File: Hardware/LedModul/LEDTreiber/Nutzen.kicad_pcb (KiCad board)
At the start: 2 copper layers, 84 x 84 mm, 400 parts, among them J1 Conn_01x01_Pin, J2 Conn_01x01_Pin, J3 Conn_01x01_Pin, J4 Conn_01x01_Pin, J5 Conn_01x01_Pin, U1 TPS92200DxRXL, U2 TVS2700DRV

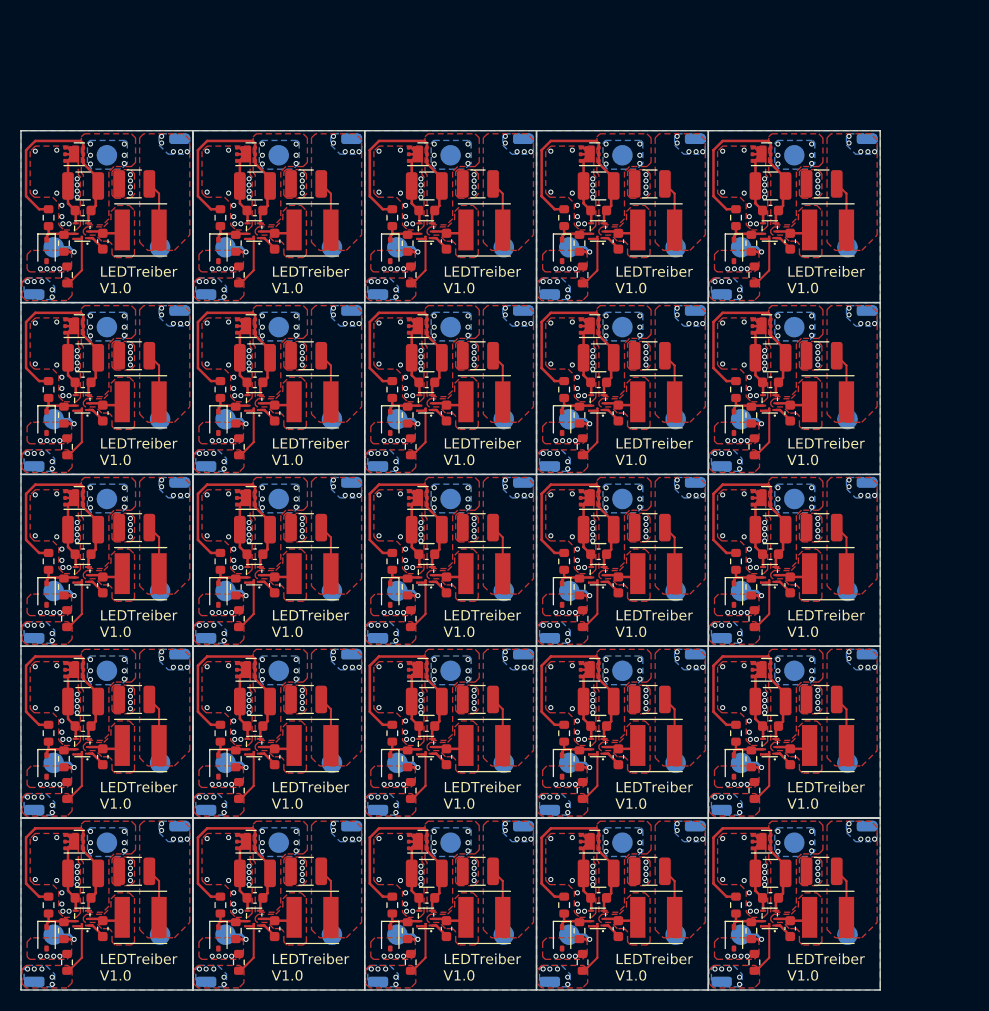
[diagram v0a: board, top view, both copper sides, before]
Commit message: V1.1
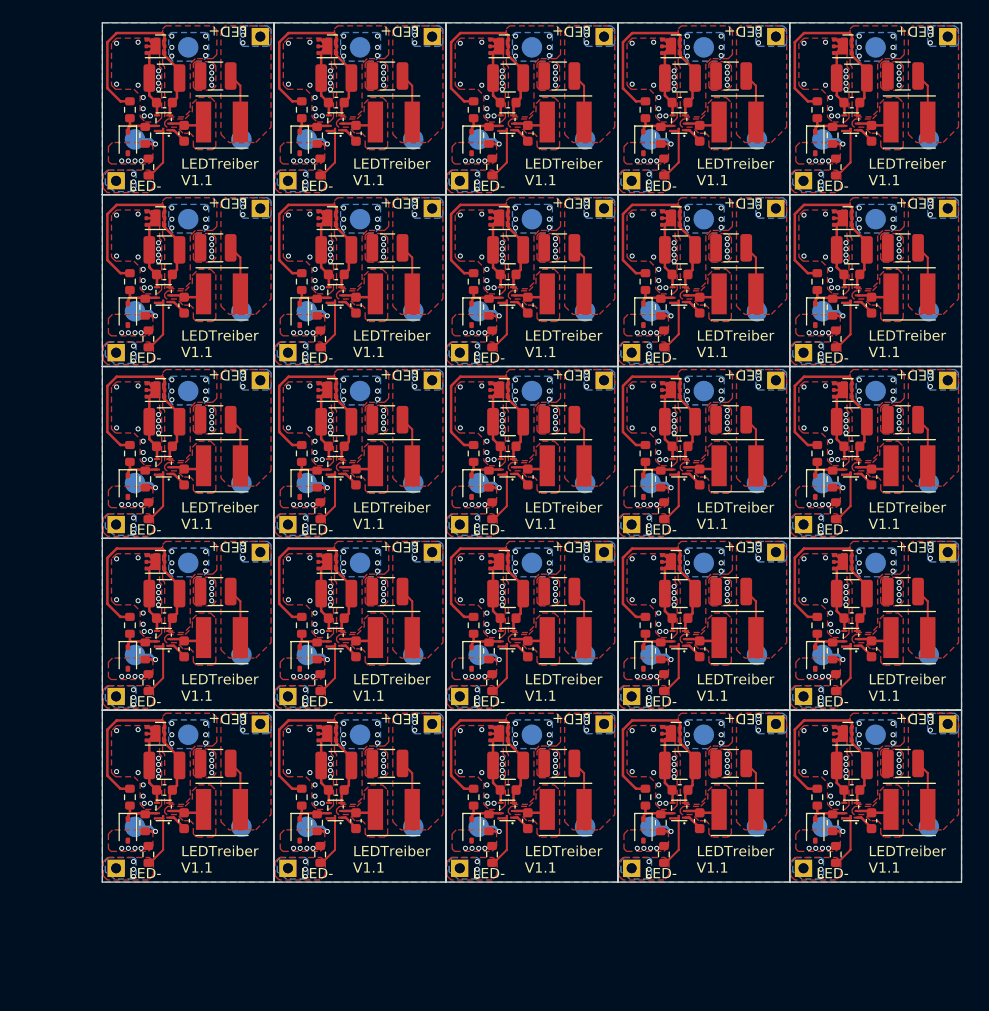
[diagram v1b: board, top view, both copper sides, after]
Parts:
- removed the C1 at (130.6, 64.8)
- removed the C1 at (97.0, 81.5)
- removed the C1 at (80.2, 115.2)
- removed the C1 at (97.0, 98.3)
- removed the C1 at (113.8, 98.3)
- removed the C1 at (147.4, 115.2)
- removed the C1 at (113.8, 64.8)
- removed the C1 at (130.6, 98.3)
- removed the C1 at (113.8, 48.0)
- removed the C1 at (80.2, 81.5)
- removed the C1 at (97.0, 64.8)
- removed the C1 at (147.4, 98.3)
- removed the C1 at (130.6, 81.5)
- removed the C1 at (147.4, 81.5)
- removed the C1 at (113.8, 115.2)
- removed the C1 at (130.6, 48.0)
- removed the C1 at (147.4, 64.8)
- removed the C1 at (147.4, 48.0)
- removed the C1 at (80.2, 98.3)
- removed the C1 at (97.0, 48.0)
- removed the C1 at (130.6, 115.2)
- removed the C1 at (80.2, 64.8)
- removed the C1 at (97.0, 115.2)
- removed the C1 at (113.8, 81.5)
- removed the C1 at (80.2, 48.0)
- removed the C2 at (110.8, 53.5)
- removed the C2 at (110.8, 120.8)
- removed the C2 at (127.5, 53.5)
- removed the C2 at (110.8, 87.2)
- removed the C2 at (110.8, 70.3)
- removed the C2 at (144.3, 53.5)
- removed the C2 at (94.0, 120.8)
- removed the C2 at (77.2, 87.2)
- removed the C2 at (77.2, 70.3)
- removed the C2 at (127.5, 104.0)
- removed the C2 at (144.3, 87.2)
- removed the C2 at (77.2, 53.5)
- removed the C2 at (94.0, 53.5)
- removed the C2 at (94.0, 104.0)
- removed the C2 at (144.3, 104.0)
- removed the C2 at (77.2, 104.0)
- removed the C2 at (127.5, 87.2)
- removed the C2 at (110.8, 104.0)
- removed the C2 at (144.3, 120.8)
- removed the C2 at (144.3, 70.3)
- removed the C2 at (94.0, 87.2)
- removed the C2 at (127.5, 70.3)
- removed the C2 at (127.5, 120.8)
- removed the C2 at (77.2, 120.8)
- removed the C2 at (94.0, 70.3)
- removed the C3 at (75.2, 115.3)
- removed the C3 at (142.4, 65.0)
- removed the C3 at (142.4, 81.8)
- removed the C3 at (75.2, 98.5)
- removed the C3 at (125.6, 98.5)
- removed the C3 at (108.8, 115.3)
- removed the C3 at (142.4, 98.5)
- removed the C3 at (75.2, 81.8)
- removed the C3 at (92.0, 98.5)
- removed the C3 at (125.6, 48.1)
- removed the C3 at (108.8, 65.0)
- removed the C3 at (142.4, 48.1)
- removed the C3 at (108.8, 81.8)
- removed the C3 at (92.0, 81.8)
- removed the C3 at (108.8, 48.1)
- removed the C3 at (125.6, 65.0)
- removed the C3 at (75.2, 48.1)
- removed the C3 at (92.0, 48.1)
- removed the C3 at (142.4, 115.3)
- removed the C3 at (125.6, 81.8)
- removed the C3 at (75.2, 65.0)
- removed the C3 at (125.6, 115.3)
- removed the C3 at (108.8, 98.5)
- removed the C3 at (92.0, 65.0)
- removed the C3 at (92.0, 115.3)
- removed the C4 at (92.0, 117.8)
- removed the C4 at (125.6, 67.3)
- removed the C4 at (142.4, 50.5)
- removed the C4 at (125.6, 101.0)
- removed the C4 at (142.4, 101.0)
- removed the C4 at (125.6, 50.5)
- removed the C4 at (108.8, 50.5)
- removed the C4 at (108.8, 84.2)
- removed the C4 at (75.2, 101.0)
- removed the C4 at (142.4, 84.2)
- removed the C4 at (142.4, 117.8)
- removed the C4 at (108.8, 67.3)
- removed the C4 at (92.0, 84.2)
- removed the C4 at (92.0, 67.3)
- removed the C4 at (75.2, 117.8)
- removed the C4 at (92.0, 101.0)
- removed the C4 at (125.6, 84.2)
- removed the C4 at (75.2, 67.3)
- removed the C4 at (75.2, 84.2)
- removed the C4 at (142.4, 67.3)
- removed the C4 at (75.2, 50.5)
- removed the C4 at (108.8, 117.8)
- removed the C4 at (108.8, 101.0)
- removed the C4 at (125.6, 117.8)
- removed the C4 at (92.0, 50.5)
- removed the D1 at (88.5, 88.0)
- removed the D1 at (71.7, 54.5)
- removed the D1 at (88.5, 71.2)
- removed the D1 at (71.7, 71.2)
- removed the D1 at (71.7, 104.8)
- removed the D1 at (88.5, 104.8)
- removed the D1 at (88.5, 54.5)
- removed the D1 at (138.8, 71.2)
- removed the D1 at (122.0, 88.0)
- removed the D1 at (88.5, 121.7)
- removed the D1 at (105.2, 121.7)
- removed the D1 at (122.0, 104.8)
- removed the D1 at (138.8, 121.7)
- removed the D1 at (71.7, 88.0)
- removed the D1 at (105.2, 71.2)
- removed the D1 at (105.2, 54.5)
- removed the D1 at (138.8, 54.5)
- removed the D1 at (122.0, 121.7)
- removed the D1 at (105.2, 88.0)
- removed the D1 at (138.8, 104.8)
- removed the D1 at (105.2, 104.8)
- removed the D1 at (122.0, 71.2)
- removed the D1 at (138.8, 88.0)
- removed the D1 at (71.7, 121.7)
- removed the D1 at (122.0, 54.5)
- removed the J1 at (118.2, 43.5)
- removed the J1 at (118.2, 110.8)
- removed the J1 at (101.5, 94.0)
- removed the J1 at (151.8, 110.8)
- removed the J1 at (84.7, 110.8)
- removed the J1 at (118.2, 60.4)
- removed the J1 at (151.8, 77.2)
- removed the J1 at (101.5, 110.8)
- removed the J1 at (135.1, 77.2)
- removed the J1 at (101.5, 60.4)
- removed the J1 at (84.7, 94.0)
- removed the J1 at (118.2, 94.0)
- removed the J1 at (151.8, 60.4)
- removed the J1 at (118.2, 77.2)
- removed the J1 at (151.8, 43.5)
- removed the J1 at (84.7, 77.2)
- removed the J1 at (101.5, 43.5)
- removed the J1 at (151.8, 94.0)
- removed the J1 at (135.1, 94.0)
- removed the J1 at (84.7, 60.4)
- removed the J1 at (135.1, 43.5)
- removed the J1 at (135.1, 110.8)
- removed the J1 at (84.7, 43.5)
- removed the J1 at (135.1, 60.4)
- removed the J1 at (101.5, 77.2)
- removed the J2 at (104.0, 58.8)
- removed the J2 at (70.5, 75.5)
- removed the J2 at (87.2, 92.3)
- removed the J2 at (104.0, 92.3)
- removed the J2 at (137.7, 126.0)
- removed the J2 at (70.5, 126.0)
- removed the J2 at (120.8, 58.8)
- removed the J2 at (104.0, 75.5)
- removed the J2 at (120.8, 75.5)
- removed the J2 at (120.8, 126.0)
- removed the J2 at (87.2, 109.2)
- removed the J2 at (137.7, 75.5)
- removed the J2 at (70.5, 58.8)
- removed the J2 at (70.5, 92.3)
- removed the J2 at (137.7, 109.2)
- removed the J2 at (120.8, 92.3)
- removed the J2 at (120.8, 109.2)
- removed the J2 at (104.0, 126.0)
- removed the J2 at (104.0, 109.2)
- removed the J2 at (87.2, 58.8)
- removed the J2 at (137.7, 58.8)
- removed the J2 at (87.2, 126.0)
- removed the J2 at (137.7, 92.3)
- removed the J2 at (87.2, 75.5)
- removed the J2 at (70.5, 109.2)
- removed the J3 at (72.3, 71.0)
- removed the J3 at (72.3, 87.8)
- removed the J3 at (89.2, 104.5)
- removed the J3 at (139.6, 54.1)
- removed the J3 at (106.0, 104.5)
- removed the J3 at (72.3, 121.3)
- removed the J3 at (106.0, 54.1)
- removed the J3 at (106.0, 121.3)
- removed the J3 at (89.2, 54.1)
- removed the J3 at (106.0, 71.0)
- removed the J3 at (89.2, 87.8)
- removed the J3 at (122.8, 104.5)
- removed the J3 at (72.3, 104.5)
- removed the J3 at (72.3, 54.1)
- removed the J3 at (139.6, 104.5)
- removed the J3 at (89.2, 121.3)
- removed the J3 at (122.8, 121.3)
- removed the J3 at (139.6, 121.3)
- removed the J3 at (122.8, 54.1)
- removed the J3 at (89.2, 71.0)
- removed the J3 at (122.8, 71.0)
- removed the J3 at (139.6, 71.0)
- removed the J3 at (139.6, 87.8)
- removed the J3 at (122.8, 87.8)
- removed the J3 at (106.0, 87.8)
- removed the J4 at (94.3, 78.8)
- removed the J4 at (144.8, 62.0)
- removed the J4 at (77.5, 95.5)
- removed the J4 at (128.0, 45.1)
- removed the J4 at (77.5, 112.3)
- removed the J4 at (77.5, 62.0)
- removed the J4 at (111.2, 62.0)
- removed the J4 at (111.2, 45.1)
- removed the J4 at (94.3, 45.1)
- removed the J4 at (128.0, 62.0)
- removed the J4 at (144.8, 95.5)
- removed the J4 at (111.2, 95.5)
- removed the J4 at (94.3, 112.3)
- removed the J4 at (94.3, 95.5)
- removed the J4 at (77.5, 78.8)
- removed the J4 at (94.3, 62.0)
- removed the J4 at (111.2, 112.3)
- removed the J4 at (128.0, 78.8)
- removed the J4 at (128.0, 95.5)
- removed the J4 at (144.8, 45.1)
- removed the J4 at (144.8, 112.3)
- removed the J4 at (128.0, 112.3)
- removed the J4 at (144.8, 78.8)
- removed the J4 at (77.5, 45.1)
- removed the J4 at (111.2, 78.8)
- removed the J5 at (82.8, 104.5)
- removed the J5 at (82.8, 54.1)
- removed the J5 at (99.5, 87.8)
- removed the J5 at (82.8, 71.0)
- removed the J5 at (116.3, 54.1)
- removed the J5 at (149.9, 71.0)
- removed the J5 at (99.5, 121.3)
- removed the J5 at (133.2, 54.1)
- removed the J5 at (82.8, 87.8)
- removed the J5 at (149.9, 121.3)
- removed the J5 at (133.2, 71.0)
- removed the J5 at (99.5, 104.5)
- removed the J5 at (133.2, 104.5)
- removed the J5 at (116.3, 104.5)
- removed the J5 at (116.3, 87.8)
- removed the J5 at (149.9, 54.1)
- removed the J5 at (99.5, 54.1)
- removed the J5 at (149.9, 87.8)
- removed the J5 at (116.3, 121.3)
- removed the J5 at (116.3, 71.0)
- removed the J5 at (99.5, 71.0)
- removed the J5 at (82.8, 121.3)
- removed the J5 at (133.2, 87.8)
- removed the J5 at (133.2, 121.3)
- removed the J5 at (149.9, 104.5)
- removed the L1 at (131.2, 86.0)
- removed the L1 at (97.7, 52.5)
- removed the L1 at (148.1, 102.8)
- removed the L1 at (80.8, 86.0)
- removed the L1 at (114.5, 86.0)
- removed the L1 at (80.8, 102.8)
- removed the L1 at (97.7, 119.7)
- removed the L1 at (148.1, 119.7)
- removed the L1 at (114.5, 69.2)
- removed the L1 at (97.7, 86.0)
- removed the L1 at (97.7, 102.8)
- removed the L1 at (114.5, 102.8)
- removed the L1 at (131.2, 69.2)
- removed the L1 at (131.2, 52.5)
- removed the L1 at (131.2, 119.7)
- removed the L1 at (148.1, 69.2)
- removed the L1 at (148.1, 52.5)
- removed the L1 at (80.8, 119.7)
- removed the L1 at (97.7, 69.2)
- removed the L1 at (114.5, 119.7)
- removed the L1 at (148.1, 86.0)
- removed the L1 at (131.2, 102.8)
- removed the L1 at (80.8, 52.5)
- removed the L1 at (114.5, 52.5)
- removed the L1 at (80.8, 69.2)
- removed the R1 at (139.1, 118.5)
- removed the R1 at (139.1, 101.7)
- removed the R1 at (88.7, 84.8)
- removed the R1 at (122.2, 51.2)
- removed the R1 at (122.2, 68.0)
- removed the R1 at (139.1, 84.8)
- removed the R1 at (71.8, 51.2)
- removed the R1 at (71.8, 118.5)
- removed the R1 at (105.5, 84.8)
- removed the R1 at (105.5, 51.2)
- removed the R1 at (139.1, 68.0)
- removed the R1 at (139.1, 51.2)
- removed the R1 at (71.8, 84.8)
- removed the R1 at (122.2, 101.7)
- removed the R1 at (122.2, 84.8)
- removed the R1 at (88.7, 51.2)
- removed the R1 at (105.5, 68.0)
- removed the R1 at (105.5, 118.5)
- removed the R1 at (88.7, 101.7)
- removed the R1 at (71.8, 101.7)
- removed the R1 at (71.8, 68.0)
- removed the R1 at (122.2, 118.5)
- removed the R1 at (88.7, 118.5)
- removed the R1 at (105.5, 101.7)
- removed the R1 at (88.7, 68.0)
- removed the R2 at (140.8, 90.5)
- removed the R2 at (73.7, 107.2)
- removed the R2 at (140.8, 107.2)
- removed the R2 at (107.2, 107.2)
- removed the R2 at (107.2, 90.5)
- removed the R2 at (107.2, 124.0)
- removed the R2 at (90.5, 73.7)
- removed the R2 at (73.7, 73.7)
- removed the R2 at (140.8, 124.0)
- removed the R2 at (90.5, 124.0)
- removed the R2 at (90.5, 56.9)
- removed the R2 at (107.2, 73.7)
- removed the R2 at (73.7, 124.0)
- removed the R2 at (90.5, 107.2)
- removed the R2 at (140.8, 73.7)
- removed the R2 at (73.7, 56.9)
- removed the R2 at (90.5, 90.5)
- removed the R2 at (73.7, 90.5)
- removed the R2 at (124.0, 56.9)
- removed the R2 at (140.8, 56.9)
- removed the R2 at (124.0, 107.2)
- removed the R2 at (124.0, 73.7)
- removed the R2 at (107.2, 56.9)
- removed the R2 at (124.0, 90.5)
- removed the R2 at (124.0, 124.0)
- removed the R3 at (107.0, 70.5)
- removed the R3 at (73.3, 121.0)
- removed the R3 at (73.3, 53.8)
- removed the R3 at (140.6, 121.0)
- removed the R3 at (90.2, 70.5)
- removed the R3 at (90.2, 104.2)
- removed the R3 at (123.8, 70.5)
- removed the R3 at (140.6, 104.2)
- removed the R3 at (140.6, 70.5)
- removed the R3 at (123.8, 104.2)
- removed the R3 at (123.8, 87.3)
- removed the R3 at (140.6, 53.8)
- removed the R3 at (90.2, 53.8)
- removed the R3 at (123.8, 53.8)
- removed the R3 at (107.0, 87.3)
- removed the R3 at (73.3, 104.2)
- removed the R3 at (107.0, 104.2)
- removed the R3 at (73.3, 70.5)
- removed the R3 at (107.0, 121.0)
- removed the R3 at (90.2, 87.3)
- removed the R3 at (123.8, 121.0)
- removed the R3 at (90.2, 121.0)
- removed the R3 at (140.6, 87.3)
- removed the R3 at (73.3, 87.3)
- removed the R3 at (107.0, 53.8)
- removed the U1 at (108.8, 69.3)
- removed the U1 at (125.5, 52.5)
- removed the U1 at (108.8, 103.0)
- removed the U1 at (142.3, 103.0)
- removed the U1 at (125.5, 86.2)
- removed the U1 at (142.3, 69.3)
- removed the U1 at (75.2, 86.2)
- removed the U1 at (92.0, 103.0)
- removed the U1 at (92.0, 52.5)
- removed the U1 at (92.0, 119.8)
- removed the U1 at (142.3, 52.5)
- removed the U1 at (75.2, 119.8)
- removed the U1 at (142.3, 86.2)
- removed the U1 at (75.2, 52.5)
- removed the U1 at (142.3, 119.8)
- removed the U1 at (75.2, 69.3)
- removed the U1 at (125.5, 119.8)
- removed the U1 at (108.8, 119.8)
- removed the U1 at (75.2, 103.0)
- removed the U1 at (92.0, 69.3)
- removed the U1 at (108.8, 86.2)
- removed the U1 at (125.5, 103.0)
- removed the U1 at (125.5, 69.3)
- removed the U1 at (92.0, 86.2)
- removed the U1 at (108.8, 52.5)
- removed the U2 at (91.2, 61.9)
- removed the U2 at (108.0, 112.2)
- removed the U2 at (91.2, 112.2)
- removed the U2 at (141.6, 112.2)
- removed the U2 at (141.6, 45.0)
- removed the U2 at (141.6, 95.5)
- removed the U2 at (124.8, 61.9)
- removed the U2 at (141.6, 78.7)
- removed the U2 at (141.6, 61.9)
- removed the U2 at (124.8, 45.0)
- removed the U2 at (108.0, 45.0)
- removed the U2 at (91.2, 95.5)
- removed the U2 at (124.8, 95.5)
- removed the U2 at (108.0, 78.7)
- removed the U2 at (91.2, 78.7)
- removed the U2 at (74.3, 61.9)
- removed the U2 at (124.8, 78.7)
- removed the U2 at (91.2, 45.0)
- removed the U2 at (108.0, 61.9)
- removed the U2 at (74.3, 78.7)
- removed the U2 at (108.0, 95.5)
- removed the U2 at (74.3, 45.0)
- removed the U2 at (124.8, 112.2)
- removed the U2 at (74.3, 95.5)
- removed the U2 at (74.3, 112.2)
- added C1: 10µ, Capacitor_SMD:C_1210_3225Metric, F.Cu at (155.4, 54.2)
- added C1: 10µ, Capacitor_SMD:C_1210_3225Metric, F.Cu at (121.8, 87.8)
- added C1: 10µ, Capacitor_SMD:C_1210_3225Metric, F.Cu at (105.0, 87.8)
- added C1: 10µ, Capacitor_SMD:C_1210_3225Metric, F.Cu at (138.6, 87.8)
- added C1: 10µ, Capacitor_SMD:C_1210_3225Metric, F.Cu at (88.2, 71.0)
- added C1: 10µ, Capacitor_SMD:C_1210_3225Metric, F.Cu at (121.8, 104.6)
- added C1: 10µ, Capacitor_SMD:C_1210_3225Metric, F.Cu at (155.4, 37.4)
- added C1: 10µ, Capacitor_SMD:C_1210_3225Metric, F.Cu at (138.6, 104.6)
- added C1: 10µ, Capacitor_SMD:C_1210_3225Metric, F.Cu at (121.8, 71.0)
- added C1: 10µ, Capacitor_SMD:C_1210_3225Metric, F.Cu at (105.0, 104.6)
- added C1: 10µ, Capacitor_SMD:C_1210_3225Metric, F.Cu at (155.4, 104.6)
- added C1: 10µ, Capacitor_SMD:C_1210_3225Metric, F.Cu at (105.0, 71.0)
- added C1: 10µ, Capacitor_SMD:C_1210_3225Metric, F.Cu at (105.0, 54.2)
- added C1: 10µ, Capacitor_SMD:C_1210_3225Metric, F.Cu at (88.2, 87.8)
- added C1: 10µ, Capacitor_SMD:C_1210_3225Metric, F.Cu at (88.2, 37.4)
- added C1: 10µ, Capacitor_SMD:C_1210_3225Metric, F.Cu at (155.4, 87.8)
- added C1: 10µ, Capacitor_SMD:C_1210_3225Metric, F.Cu at (88.2, 104.6)
- added C1: 10µ, Capacitor_SMD:C_1210_3225Metric, F.Cu at (155.4, 71.0)
- added C1: 10µ, Capacitor_SMD:C_1210_3225Metric, F.Cu at (138.6, 37.4)
- added C1: 10µ, Capacitor_SMD:C_1210_3225Metric, F.Cu at (138.6, 71.0)
- added C1: 10µ, Capacitor_SMD:C_1210_3225Metric, F.Cu at (105.0, 37.4)
- added C1: 10µ, Capacitor_SMD:C_1210_3225Metric, F.Cu at (121.8, 54.2)
- added C1: 10µ, Capacitor_SMD:C_1210_3225Metric, F.Cu at (138.6, 54.2)
- added C1: 10µ, Capacitor_SMD:C_1210_3225Metric, F.Cu at (88.2, 54.2)
- added C1: 10µ, Capacitor_SMD:C_1210_3225Metric, F.Cu at (121.8, 37.4)
- added C2: 100n, Capacitor_SMD:C_0603_1608Metric, F.Cu at (152.3, 93.4)
- added C2: 100n, Capacitor_SMD:C_0603_1608Metric, F.Cu at (101.9, 76.6)
- added C2: 100n, Capacitor_SMD:C_0603_1608Metric, F.Cu at (101.9, 110.2)
- added C2: 100n, Capacitor_SMD:C_0603_1608Metric, F.Cu at (101.9, 59.8)
- added C2: 100n, Capacitor_SMD:C_0603_1608Metric, F.Cu at (101.9, 93.4)
- added C2: 100n, Capacitor_SMD:C_0603_1608Metric, F.Cu at (135.5, 93.4)
- added C2: 100n, Capacitor_SMD:C_0603_1608Metric, F.Cu at (85.1, 93.4)
- added C2: 100n, Capacitor_SMD:C_0603_1608Metric, F.Cu at (152.3, 59.8)
- added C2: 100n, Capacitor_SMD:C_0603_1608Metric, F.Cu at (85.1, 76.6)
- added C2: 100n, Capacitor_SMD:C_0603_1608Metric, F.Cu at (85.1, 59.8)
- added C2: 100n, Capacitor_SMD:C_0603_1608Metric, F.Cu at (101.9, 43.0)
- added C2: 100n, Capacitor_SMD:C_0603_1608Metric, F.Cu at (118.7, 93.4)
- added C2: 100n, Capacitor_SMD:C_0603_1608Metric, F.Cu at (118.7, 110.2)
- added C2: 100n, Capacitor_SMD:C_0603_1608Metric, F.Cu at (135.5, 59.8)
- added C2: 100n, Capacitor_SMD:C_0603_1608Metric, F.Cu at (135.5, 110.2)
- added C2: 100n, Capacitor_SMD:C_0603_1608Metric, F.Cu at (118.7, 76.6)
- added C2: 100n, Capacitor_SMD:C_0603_1608Metric, F.Cu at (118.7, 43.0)
- added C2: 100n, Capacitor_SMD:C_0603_1608Metric, F.Cu at (135.5, 43.0)
- added C2: 100n, Capacitor_SMD:C_0603_1608Metric, F.Cu at (152.3, 110.2)
- added C2: 100n, Capacitor_SMD:C_0603_1608Metric, F.Cu at (152.3, 43.0)
- added C2: 100n, Capacitor_SMD:C_0603_1608Metric, F.Cu at (85.1, 110.2)
- added C2: 100n, Capacitor_SMD:C_0603_1608Metric, F.Cu at (85.1, 43.0)
- added C2: 100n, Capacitor_SMD:C_0603_1608Metric, F.Cu at (118.7, 59.8)
- added C2: 100n, Capacitor_SMD:C_0603_1608Metric, F.Cu at (152.3, 76.6)
- added C2: 100n, Capacitor_SMD:C_0603_1608Metric, F.Cu at (135.5, 76.6)
- added C3: 10µ, Capacitor_SMD:C_1210_3225Metric, F.Cu at (133.6, 54.4)
- added C3: 10µ, Capacitor_SMD:C_1210_3225Metric, F.Cu at (116.8, 71.2)
- added C3: 10µ, Capacitor_SMD:C_1210_3225Metric, F.Cu at (83.2, 71.2)
- added C3: 10µ, Capacitor_SMD:C_1210_3225Metric, F.Cu at (150.4, 88.0)
- added C3: 10µ, Capacitor_SMD:C_1210_3225Metric, F.Cu at (116.8, 54.4)
- added C3: 10µ, Capacitor_SMD:C_1210_3225Metric, F.Cu at (150.4, 37.6)
- added C3: 10µ, Capacitor_SMD:C_1210_3225Metric, F.Cu at (83.2, 37.6)
- added C3: 10µ, Capacitor_SMD:C_1210_3225Metric, F.Cu at (150.4, 71.2)
- added C3: 10µ, Capacitor_SMD:C_1210_3225Metric, F.Cu at (100.0, 37.6)
- added C3: 10µ, Capacitor_SMD:C_1210_3225Metric, F.Cu at (133.6, 71.2)
- added C3: 10µ, Capacitor_SMD:C_1210_3225Metric, F.Cu at (83.2, 88.0)
- added C3: 10µ, Capacitor_SMD:C_1210_3225Metric, F.Cu at (100.0, 104.8)
- added C3: 10µ, Capacitor_SMD:C_1210_3225Metric, F.Cu at (133.6, 88.0)
- added C3: 10µ, Capacitor_SMD:C_1210_3225Metric, F.Cu at (133.6, 104.8)
- added C3: 10µ, Capacitor_SMD:C_1210_3225Metric, F.Cu at (100.0, 54.4)
- added C3: 10µ, Capacitor_SMD:C_1210_3225Metric, F.Cu at (100.0, 88.0)
- added C3: 10µ, Capacitor_SMD:C_1210_3225Metric, F.Cu at (116.8, 104.8)
- added C3: 10µ, Capacitor_SMD:C_1210_3225Metric, F.Cu at (133.6, 37.6)
- added C3: 10µ, Capacitor_SMD:C_1210_3225Metric, F.Cu at (83.2, 54.4)
- added C3: 10µ, Capacitor_SMD:C_1210_3225Metric, F.Cu at (100.0, 71.2)
- added C3: 10µ, Capacitor_SMD:C_1210_3225Metric, F.Cu at (150.4, 54.4)
- added C3: 10µ, Capacitor_SMD:C_1210_3225Metric, F.Cu at (83.2, 104.8)
- added C3: 10µ, Capacitor_SMD:C_1210_3225Metric, F.Cu at (150.4, 104.8)
- added C3: 10µ, Capacitor_SMD:C_1210_3225Metric, F.Cu at (116.8, 37.6)
- added C3: 10µ, Capacitor_SMD:C_1210_3225Metric, F.Cu at (116.8, 88.0)
- added C4: 100n, Capacitor_SMD:C_0603_1608Metric, F.Cu at (150.4, 56.8)
- added C4: 100n, Capacitor_SMD:C_0603_1608Metric, F.Cu at (116.8, 73.6)
- added C4: 100n, Capacitor_SMD:C_0603_1608Metric, F.Cu at (100.0, 73.6)
- added C4: 100n, Capacitor_SMD:C_0603_1608Metric, F.Cu at (133.6, 56.8)
- added C4: 100n, Capacitor_SMD:C_0603_1608Metric, F.Cu at (116.8, 107.2)
- added C4: 100n, Capacitor_SMD:C_0603_1608Metric, F.Cu at (100.0, 40.0)
- added C4: 100n, Capacitor_SMD:C_0603_1608Metric, F.Cu at (83.2, 40.0)
- added C4: 100n, Capacitor_SMD:C_0603_1608Metric, F.Cu at (116.8, 90.4)
- added C4: 100n, Capacitor_SMD:C_0603_1608Metric, F.Cu at (133.6, 73.6)
- added C4: 100n, Capacitor_SMD:C_0603_1608Metric, F.Cu at (116.8, 56.8)
- added C4: 100n, Capacitor_SMD:C_0603_1608Metric, F.Cu at (150.4, 73.6)
- added C4: 100n, Capacitor_SMD:C_0603_1608Metric, F.Cu at (150.4, 90.4)
- added C4: 100n, Capacitor_SMD:C_0603_1608Metric, F.Cu at (100.0, 56.8)
- added C4: 100n, Capacitor_SMD:C_0603_1608Metric, F.Cu at (100.0, 90.4)
- added C4: 100n, Capacitor_SMD:C_0603_1608Metric, F.Cu at (150.4, 107.2)
- added C4: 100n, Capacitor_SMD:C_0603_1608Metric, F.Cu at (100.0, 107.2)
- added C4: 100n, Capacitor_SMD:C_0603_1608Metric, F.Cu at (83.2, 90.4)
- added C4: 100n, Capacitor_SMD:C_0603_1608Metric, F.Cu at (133.6, 90.4)
- added C4: 100n, Capacitor_SMD:C_0603_1608Metric, F.Cu at (150.4, 40.0)
- added C4: 100n, Capacitor_SMD:C_0603_1608Metric, F.Cu at (83.2, 107.2)
- added C4: 100n, Capacitor_SMD:C_0603_1608Metric, F.Cu at (133.6, 40.0)
- added C4: 100n, Capacitor_SMD:C_0603_1608Metric, F.Cu at (133.6, 107.2)
- added C4: 100n, Capacitor_SMD:C_0603_1608Metric, F.Cu at (83.2, 56.8)
- added C4: 100n, Capacitor_SMD:C_0603_1608Metric, F.Cu at (116.8, 40.0)
- added C4: 100n, Capacitor_SMD:C_0603_1608Metric, F.Cu at (83.2, 73.6)
- added D1: 3V3, Diode_SMD:D_SOD-323, F.Cu at (130.0, 111.1)
- added D1: 3V3, Diode_SMD:D_SOD-323, F.Cu at (79.6, 60.7)
- added D1: 3V3, Diode_SMD:D_SOD-323, F.Cu at (113.2, 94.3)
- added D1: 3V3, Diode_SMD:D_SOD-323, F.Cu at (96.4, 77.5)
- added D1: 3V3, Diode_SMD:D_SOD-323, F.Cu at (113.2, 43.9)
- added D1: 3V3, Diode_SMD:D_SOD-323, F.Cu at (146.8, 60.7)
- added D1: 3V3, Diode_SMD:D_SOD-323, F.Cu at (96.4, 94.3)
- added D1: 3V3, Diode_SMD:D_SOD-323, F.Cu at (130.0, 77.5)
- added D1: 3V3, Diode_SMD:D_SOD-323, F.Cu at (146.8, 111.1)
- added D1: 3V3, Diode_SMD:D_SOD-323, F.Cu at (96.4, 111.1)
- added D1: 3V3, Diode_SMD:D_SOD-323, F.Cu at (146.8, 77.5)
- added D1: 3V3, Diode_SMD:D_SOD-323, F.Cu at (79.6, 94.3)
- added D1: 3V3, Diode_SMD:D_SOD-323, F.Cu at (79.6, 43.9)
- added D1: 3V3, Diode_SMD:D_SOD-323, F.Cu at (146.8, 94.3)
- added D1: 3V3, Diode_SMD:D_SOD-323, F.Cu at (146.8, 43.9)
- added D1: 3V3, Diode_SMD:D_SOD-323, F.Cu at (79.6, 77.5)
- added D1: 3V3, Diode_SMD:D_SOD-323, F.Cu at (130.0, 43.9)
- added D1: 3V3, Diode_SMD:D_SOD-323, F.Cu at (96.4, 43.9)
- added D1: 3V3, Diode_SMD:D_SOD-323, F.Cu at (113.2, 111.1)
- added D1: 3V3, Diode_SMD:D_SOD-323, F.Cu at (113.2, 77.5)
- added D1: 3V3, Diode_SMD:D_SOD-323, F.Cu at (79.6, 111.1)
- added D1: 3V3, Diode_SMD:D_SOD-323, F.Cu at (113.2, 60.7)
- added D1: 3V3, Diode_SMD:D_SOD-323, F.Cu at (96.4, 60.7)
- added D1: 3V3, Diode_SMD:D_SOD-323, F.Cu at (130.0, 94.3)
- added D1: 3V3, Diode_SMD:D_SOD-323, F.Cu at (130.0, 60.7)
- added J1: Conn_01x01_Pin, Connector_PinHeader_2.54mm:PinHeader_1x01_P2.54mm_Vertical, F.Cu at (159.8, 50.4)
- added J1: Conn_01x01_Pin, Connector_PinHeader_2.54mm:PinHeader_1x01_P2.54mm_Vertical, F.Cu at (109.3, 100.8)
- added J1: Conn_01x01_Pin, Connector_PinHeader_2.54mm:PinHeader_1x01_P2.54mm_Vertical, F.Cu at (92.5, 67.2)
- added J1: Conn_01x01_Pin, Connector_PinHeader_2.54mm:PinHeader_1x01_P2.54mm_Vertical, F.Cu at (92.5, 50.4)
- added J1: Conn_01x01_Pin, Connector_PinHeader_2.54mm:PinHeader_1x01_P2.54mm_Vertical, F.Cu at (159.8, 84.0)
- added J1: Conn_01x01_Pin, Connector_PinHeader_2.54mm:PinHeader_1x01_P2.54mm_Vertical, F.Cu at (109.3, 33.5)
- added J1: Conn_01x01_Pin, Connector_PinHeader_2.54mm:PinHeader_1x01_P2.54mm_Vertical, F.Cu at (159.8, 67.2)
- added J1: Conn_01x01_Pin, Connector_PinHeader_2.54mm:PinHeader_1x01_P2.54mm_Vertical, F.Cu at (126.2, 50.4)
- added J1: Conn_01x01_Pin, Connector_PinHeader_2.54mm:PinHeader_1x01_P2.54mm_Vertical, F.Cu at (126.2, 33.5)
- added J1: Conn_01x01_Pin, Connector_PinHeader_2.54mm:PinHeader_1x01_P2.54mm_Vertical, F.Cu at (142.9, 100.8)
- added J1: Conn_01x01_Pin, Connector_PinHeader_2.54mm:PinHeader_1x01_P2.54mm_Vertical, F.Cu at (109.3, 50.4)
- added J1: Conn_01x01_Pin, Connector_PinHeader_2.54mm:PinHeader_1x01_P2.54mm_Vertical, F.Cu at (126.2, 67.2)
- added J1: Conn_01x01_Pin, Connector_PinHeader_2.54mm:PinHeader_1x01_P2.54mm_Vertical, F.Cu at (92.5, 100.8)
- added J1: Conn_01x01_Pin, Connector_PinHeader_2.54mm:PinHeader_1x01_P2.54mm_Vertical, F.Cu at (126.2, 100.8)
- added J1: Conn_01x01_Pin, Connector_PinHeader_2.54mm:PinHeader_1x01_P2.54mm_Vertical, F.Cu at (159.8, 100.8)
- added J1: Conn_01x01_Pin, Connector_PinHeader_2.54mm:PinHeader_1x01_P2.54mm_Vertical, F.Cu at (142.9, 33.5)
- added J1: Conn_01x01_Pin, Connector_PinHeader_2.54mm:PinHeader_1x01_P2.54mm_Vertical, F.Cu at (109.3, 67.2)
- added J1: Conn_01x01_Pin, Connector_PinHeader_2.54mm:PinHeader_1x01_P2.54mm_Vertical, F.Cu at (159.8, 33.5)
- added J1: Conn_01x01_Pin, Connector_PinHeader_2.54mm:PinHeader_1x01_P2.54mm_Vertical, F.Cu at (109.3, 84.0)
- added J1: Conn_01x01_Pin, Connector_PinHeader_2.54mm:PinHeader_1x01_P2.54mm_Vertical, F.Cu at (142.9, 84.0)
- added J1: Conn_01x01_Pin, Connector_PinHeader_2.54mm:PinHeader_1x01_P2.54mm_Vertical, F.Cu at (142.9, 50.4)
- added J1: Conn_01x01_Pin, Connector_PinHeader_2.54mm:PinHeader_1x01_P2.54mm_Vertical, F.Cu at (92.5, 84.0)
- added J1: Conn_01x01_Pin, Connector_PinHeader_2.54mm:PinHeader_1x01_P2.54mm_Vertical, F.Cu at (126.2, 84.0)
- added J1: Conn_01x01_Pin, Connector_PinHeader_2.54mm:PinHeader_1x01_P2.54mm_Vertical, F.Cu at (142.9, 67.2)
- added J1: Conn_01x01_Pin, Connector_PinHeader_2.54mm:PinHeader_1x01_P2.54mm_Vertical, F.Cu at (92.5, 33.5)
- added J2: Conn_01x01_Pin, Connector_PinHeader_2.54mm:PinHeader_1x01_P2.54mm_Vertical, F.Cu at (95.2, 114.8)
- added J2: Conn_01x01_Pin, Connector_PinHeader_2.54mm:PinHeader_1x01_P2.54mm_Vertical, F.Cu at (145.7, 81.2)
- added J2: Conn_01x01_Pin, Connector_PinHeader_2.54mm:PinHeader_1x01_P2.54mm_Vertical, F.Cu at (112.0, 64.5)
- added J2: Conn_01x01_Pin, Connector_PinHeader_2.54mm:PinHeader_1x01_P2.54mm_Vertical, F.Cu at (112.0, 114.8)
- added J2: Conn_01x01_Pin, Connector_PinHeader_2.54mm:PinHeader_1x01_P2.54mm_Vertical, F.Cu at (128.8, 98.0)
- added J2: Conn_01x01_Pin, Connector_PinHeader_2.54mm:PinHeader_1x01_P2.54mm_Vertical, F.Cu at (145.7, 114.8)
- added J2: Conn_01x01_Pin, Connector_PinHeader_2.54mm:PinHeader_1x01_P2.54mm_Vertical, F.Cu at (95.2, 98.0)
- added J2: Conn_01x01_Pin, Connector_PinHeader_2.54mm:PinHeader_1x01_P2.54mm_Vertical, F.Cu at (95.2, 64.5)
- added J2: Conn_01x01_Pin, Connector_PinHeader_2.54mm:PinHeader_1x01_P2.54mm_Vertical, F.Cu at (145.7, 98.0)
- added J2: Conn_01x01_Pin, Connector_PinHeader_2.54mm:PinHeader_1x01_P2.54mm_Vertical, F.Cu at (78.5, 114.8)
- added J2: Conn_01x01_Pin, Connector_PinHeader_2.54mm:PinHeader_1x01_P2.54mm_Vertical, F.Cu at (128.8, 114.8)
- added J2: Conn_01x01_Pin, Connector_PinHeader_2.54mm:PinHeader_1x01_P2.54mm_Vertical, F.Cu at (128.8, 64.5)
- added J2: Conn_01x01_Pin, Connector_PinHeader_2.54mm:PinHeader_1x01_P2.54mm_Vertical, F.Cu at (78.5, 47.6)
- added J2: Conn_01x01_Pin, Connector_PinHeader_2.54mm:PinHeader_1x01_P2.54mm_Vertical, F.Cu at (95.2, 81.2)
- added J2: Conn_01x01_Pin, Connector_PinHeader_2.54mm:PinHeader_1x01_P2.54mm_Vertical, F.Cu at (78.5, 81.2)
- added J2: Conn_01x01_Pin, Connector_PinHeader_2.54mm:PinHeader_1x01_P2.54mm_Vertical, F.Cu at (112.0, 81.2)
- added J2: Conn_01x01_Pin, Connector_PinHeader_2.54mm:PinHeader_1x01_P2.54mm_Vertical, F.Cu at (78.5, 64.5)
- added J2: Conn_01x01_Pin, Connector_PinHeader_2.54mm:PinHeader_1x01_P2.54mm_Vertical, F.Cu at (112.0, 98.0)
- added J2: Conn_01x01_Pin, Connector_PinHeader_2.54mm:PinHeader_1x01_P2.54mm_Vertical, F.Cu at (128.8, 47.6)
- added J2: Conn_01x01_Pin, Connector_PinHeader_2.54mm:PinHeader_1x01_P2.54mm_Vertical, F.Cu at (78.5, 98.0)
- added J2: Conn_01x01_Pin, Connector_PinHeader_2.54mm:PinHeader_1x01_P2.54mm_Vertical, F.Cu at (145.7, 64.5)
- added J2: Conn_01x01_Pin, Connector_PinHeader_2.54mm:PinHeader_1x01_P2.54mm_Vertical, F.Cu at (145.7, 47.6)
- added J2: Conn_01x01_Pin, Connector_PinHeader_2.54mm:PinHeader_1x01_P2.54mm_Vertical, F.Cu at (95.2, 47.6)
- added J2: Conn_01x01_Pin, Connector_PinHeader_2.54mm:PinHeader_1x01_P2.54mm_Vertical, F.Cu at (128.8, 81.2)
- added J2: Conn_01x01_Pin, Connector_PinHeader_2.54mm:PinHeader_1x01_P2.54mm_Vertical, F.Cu at (112.0, 47.6)
- added J3: Conn_01x01_Pin, TestPoint:TestPoint_Pad_D2.0mm, B.Cu at (113.9, 43.6)
- added J3: Conn_01x01_Pin, TestPoint:TestPoint_Pad_D2.0mm, B.Cu at (130.7, 110.8)
- added J3: Conn_01x01_Pin, TestPoint:TestPoint_Pad_D2.0mm, B.Cu at (113.9, 77.2)
- added J3: Conn_01x01_Pin, TestPoint:TestPoint_Pad_D2.0mm, B.Cu at (80.3, 60.4)
- added J3: Conn_01x01_Pin, TestPoint:TestPoint_Pad_D2.0mm, B.Cu at (80.3, 77.2)
- added J3: Conn_01x01_Pin, TestPoint:TestPoint_Pad_D2.0mm, B.Cu at (130.7, 43.6)
- added J3: Conn_01x01_Pin, TestPoint:TestPoint_Pad_D2.0mm, B.Cu at (80.3, 110.8)
- added J3: Conn_01x01_Pin, TestPoint:TestPoint_Pad_D2.0mm, B.Cu at (113.9, 60.4)
- added J3: Conn_01x01_Pin, TestPoint:TestPoint_Pad_D2.0mm, B.Cu at (130.7, 77.2)
- added J3: Conn_01x01_Pin, TestPoint:TestPoint_Pad_D2.0mm, B.Cu at (147.5, 77.2)
- added J3: Conn_01x01_Pin, TestPoint:TestPoint_Pad_D2.0mm, B.Cu at (147.5, 60.4)
- added J3: Conn_01x01_Pin, TestPoint:TestPoint_Pad_D2.0mm, B.Cu at (113.9, 94.0)
- added J3: Conn_01x01_Pin, TestPoint:TestPoint_Pad_D2.0mm, B.Cu at (130.7, 94.0)
- added J3: Conn_01x01_Pin, TestPoint:TestPoint_Pad_D2.0mm, B.Cu at (147.5, 110.8)
- added J3: Conn_01x01_Pin, TestPoint:TestPoint_Pad_D2.0mm, B.Cu at (97.1, 60.4)
- added J3: Conn_01x01_Pin, TestPoint:TestPoint_Pad_D2.0mm, B.Cu at (147.5, 94.0)
- added J3: Conn_01x01_Pin, TestPoint:TestPoint_Pad_D2.0mm, B.Cu at (130.7, 60.4)
- added J3: Conn_01x01_Pin, TestPoint:TestPoint_Pad_D2.0mm, B.Cu at (97.1, 43.6)
- added J3: Conn_01x01_Pin, TestPoint:TestPoint_Pad_D2.0mm, B.Cu at (113.9, 110.8)
- added J3: Conn_01x01_Pin, TestPoint:TestPoint_Pad_D2.0mm, B.Cu at (80.3, 43.6)
- added J3: Conn_01x01_Pin, TestPoint:TestPoint_Pad_D2.0mm, B.Cu at (147.5, 43.6)
- added J3: Conn_01x01_Pin, TestPoint:TestPoint_Pad_D2.0mm, B.Cu at (80.3, 94.0)
- added J3: Conn_01x01_Pin, TestPoint:TestPoint_Pad_D2.0mm, B.Cu at (97.1, 110.8)
- added J3: Conn_01x01_Pin, TestPoint:TestPoint_Pad_D2.0mm, B.Cu at (97.1, 77.2)
- added J3: Conn_01x01_Pin, TestPoint:TestPoint_Pad_D2.0mm, B.Cu at (97.1, 94.0)
- added J4: Conn_01x01_Pin, TestPoint:TestPoint_Pad_D2.0mm, B.Cu at (119.1, 85.0)
- added J4: Conn_01x01_Pin, TestPoint:TestPoint_Pad_D2.0mm, B.Cu at (85.5, 51.4)
- added J4: Conn_01x01_Pin, TestPoint:TestPoint_Pad_D2.0mm, B.Cu at (102.3, 85.0)
- added J4: Conn_01x01_Pin, TestPoint:TestPoint_Pad_D2.0mm, B.Cu at (102.3, 68.2)
- added J4: Conn_01x01_Pin, TestPoint:TestPoint_Pad_D2.0mm, B.Cu at (85.5, 68.2)
- added J4: Conn_01x01_Pin, TestPoint:TestPoint_Pad_D2.0mm, B.Cu at (85.5, 34.6)
- added J4: Conn_01x01_Pin, TestPoint:TestPoint_Pad_D2.0mm, B.Cu at (119.1, 34.6)
- added J4: Conn_01x01_Pin, TestPoint:TestPoint_Pad_D2.0mm, B.Cu at (152.7, 68.2)
- added J4: Conn_01x01_Pin, TestPoint:TestPoint_Pad_D2.0mm, B.Cu at (135.9, 34.6)
- added J4: Conn_01x01_Pin, TestPoint:TestPoint_Pad_D2.0mm, B.Cu at (119.1, 51.4)
- added J4: Conn_01x01_Pin, TestPoint:TestPoint_Pad_D2.0mm, B.Cu at (85.5, 85.0)
- added J4: Conn_01x01_Pin, TestPoint:TestPoint_Pad_D2.0mm, B.Cu at (135.9, 85.0)
- added J4: Conn_01x01_Pin, TestPoint:TestPoint_Pad_D2.0mm, B.Cu at (102.3, 51.4)
- added J4: Conn_01x01_Pin, TestPoint:TestPoint_Pad_D2.0mm, B.Cu at (135.9, 51.4)
- added J4: Conn_01x01_Pin, TestPoint:TestPoint_Pad_D2.0mm, B.Cu at (135.9, 68.2)
- added J4: Conn_01x01_Pin, TestPoint:TestPoint_Pad_D2.0mm, B.Cu at (102.3, 34.6)
- added J4: Conn_01x01_Pin, TestPoint:TestPoint_Pad_D2.0mm, B.Cu at (119.1, 68.2)
- added J4: Conn_01x01_Pin, TestPoint:TestPoint_Pad_D2.0mm, B.Cu at (152.7, 51.4)
- added J4: Conn_01x01_Pin, TestPoint:TestPoint_Pad_D2.0mm, B.Cu at (119.1, 101.8)
- added J4: Conn_01x01_Pin, TestPoint:TestPoint_Pad_D2.0mm, B.Cu at (102.3, 101.8)
- added J4: Conn_01x01_Pin, TestPoint:TestPoint_Pad_D2.0mm, B.Cu at (152.7, 34.6)
- added J4: Conn_01x01_Pin, TestPoint:TestPoint_Pad_D2.0mm, B.Cu at (135.9, 101.8)
- added J4: Conn_01x01_Pin, TestPoint:TestPoint_Pad_D2.0mm, B.Cu at (85.5, 101.8)
- added J4: Conn_01x01_Pin, TestPoint:TestPoint_Pad_D2.0mm, B.Cu at (152.7, 85.0)
- added J4: Conn_01x01_Pin, TestPoint:TestPoint_Pad_D2.0mm, B.Cu at (152.7, 101.8)
- added J5: Conn_01x01_Pin, TestPoint:TestPoint_Pad_D2.0mm, B.Cu at (107.5, 60.4)
- added J5: Conn_01x01_Pin, TestPoint:TestPoint_Pad_D2.0mm, B.Cu at (141.1, 94.0)
- added J5: Conn_01x01_Pin, TestPoint:TestPoint_Pad_D2.0mm, B.Cu at (157.9, 43.6)
- added J5: Conn_01x01_Pin, TestPoint:TestPoint_Pad_D2.0mm, B.Cu at (90.7, 60.4)
- added J5: Conn_01x01_Pin, TestPoint:TestPoint_Pad_D2.0mm, B.Cu at (157.9, 110.8)
- added J5: Conn_01x01_Pin, TestPoint:TestPoint_Pad_D2.0mm, B.Cu at (141.1, 60.4)
- added J5: Conn_01x01_Pin, TestPoint:TestPoint_Pad_D2.0mm, B.Cu at (141.1, 110.8)
- added J5: Conn_01x01_Pin, TestPoint:TestPoint_Pad_D2.0mm, B.Cu at (124.3, 110.8)
- added J5: Conn_01x01_Pin, TestPoint:TestPoint_Pad_D2.0mm, B.Cu at (107.5, 94.0)
- added J5: Conn_01x01_Pin, TestPoint:TestPoint_Pad_D2.0mm, B.Cu at (107.5, 43.6)
- added J5: Conn_01x01_Pin, TestPoint:TestPoint_Pad_D2.0mm, B.Cu at (157.9, 77.2)
- added J5: Conn_01x01_Pin, TestPoint:TestPoint_Pad_D2.0mm, B.Cu at (90.7, 43.6)
- added J5: Conn_01x01_Pin, TestPoint:TestPoint_Pad_D2.0mm, B.Cu at (124.3, 43.6)
- added J5: Conn_01x01_Pin, TestPoint:TestPoint_Pad_D2.0mm, B.Cu at (124.3, 94.0)
- added J5: Conn_01x01_Pin, TestPoint:TestPoint_Pad_D2.0mm, B.Cu at (107.5, 110.8)
- added J5: Conn_01x01_Pin, TestPoint:TestPoint_Pad_D2.0mm, B.Cu at (141.1, 77.2)
- added J5: Conn_01x01_Pin, TestPoint:TestPoint_Pad_D2.0mm, B.Cu at (90.7, 94.0)
- added J5: Conn_01x01_Pin, TestPoint:TestPoint_Pad_D2.0mm, B.Cu at (124.3, 77.2)
- added J5: Conn_01x01_Pin, TestPoint:TestPoint_Pad_D2.0mm, B.Cu at (90.7, 110.8)
- added J5: Conn_01x01_Pin, TestPoint:TestPoint_Pad_D2.0mm, B.Cu at (124.3, 60.4)
- added J5: Conn_01x01_Pin, TestPoint:TestPoint_Pad_D2.0mm, B.Cu at (107.5, 77.2)
- added J5: Conn_01x01_Pin, TestPoint:TestPoint_Pad_D2.0mm, B.Cu at (157.9, 94.0)
- added J5: Conn_01x01_Pin, TestPoint:TestPoint_Pad_D2.0mm, B.Cu at (157.9, 60.4)
- added J5: Conn_01x01_Pin, TestPoint:TestPoint_Pad_D2.0mm, B.Cu at (90.7, 77.2)
- added J5: Conn_01x01_Pin, TestPoint:TestPoint_Pad_D2.0mm, B.Cu at (141.1, 43.6)
- added L1: 15µH, Inductor_SMD:L_Taiyo-Yuden_NR-50xx, F.Cu at (122.4, 92.3)
- added L1: 15µH, Inductor_SMD:L_Taiyo-Yuden_NR-50xx, F.Cu at (105.6, 58.7)
- added L1: 15µH, Inductor_SMD:L_Taiyo-Yuden_NR-50xx, F.Cu at (139.2, 41.9)
- added L1: 15µH, Inductor_SMD:L_Taiyo-Yuden_NR-50xx, F.Cu at (156.0, 75.5)
- added L1: 15µH, Inductor_SMD:L_Taiyo-Yuden_NR-50xx, F.Cu at (88.8, 58.7)
- added L1: 15µH, Inductor_SMD:L_Taiyo-Yuden_NR-50xx, F.Cu at (139.2, 58.7)
- added L1: 15µH, Inductor_SMD:L_Taiyo-Yuden_NR-50xx, F.Cu at (156.0, 109.1)
- added L1: 15µH, Inductor_SMD:L_Taiyo-Yuden_NR-50xx, F.Cu at (156.0, 41.9)
- added L1: 15µH, Inductor_SMD:L_Taiyo-Yuden_NR-50xx, F.Cu at (105.6, 109.1)
- added L1: 15µH, Inductor_SMD:L_Taiyo-Yuden_NR-50xx, F.Cu at (156.0, 92.3)
- added L1: 15µH, Inductor_SMD:L_Taiyo-Yuden_NR-50xx, F.Cu at (88.8, 75.5)
- added L1: 15µH, Inductor_SMD:L_Taiyo-Yuden_NR-50xx, F.Cu at (88.8, 109.1)
- added L1: 15µH, Inductor_SMD:L_Taiyo-Yuden_NR-50xx, F.Cu at (105.6, 92.3)
- added L1: 15µH, Inductor_SMD:L_Taiyo-Yuden_NR-50xx, F.Cu at (122.4, 75.5)
- added L1: 15µH, Inductor_SMD:L_Taiyo-Yuden_NR-50xx, F.Cu at (105.6, 75.5)
- added L1: 15µH, Inductor_SMD:L_Taiyo-Yuden_NR-50xx, F.Cu at (122.4, 41.9)
- added L1: 15µH, Inductor_SMD:L_Taiyo-Yuden_NR-50xx, F.Cu at (156.0, 58.7)
- added L1: 15µH, Inductor_SMD:L_Taiyo-Yuden_NR-50xx, F.Cu at (105.6, 41.9)
- added L1: 15µH, Inductor_SMD:L_Taiyo-Yuden_NR-50xx, F.Cu at (88.8, 41.9)
- added L1: 15µH, Inductor_SMD:L_Taiyo-Yuden_NR-50xx, F.Cu at (88.8, 92.3)
- added L1: 15µH, Inductor_SMD:L_Taiyo-Yuden_NR-50xx, F.Cu at (139.2, 75.5)
- added L1: 15µH, Inductor_SMD:L_Taiyo-Yuden_NR-50xx, F.Cu at (122.4, 58.7)
- added L1: 15µH, Inductor_SMD:L_Taiyo-Yuden_NR-50xx, F.Cu at (122.4, 109.1)
- added L1: 15µH, Inductor_SMD:L_Taiyo-Yuden_NR-50xx, F.Cu at (139.2, 92.3)
- added L1: 15µH, Inductor_SMD:L_Taiyo-Yuden_NR-50xx, F.Cu at (139.2, 109.1)
- added R1: 1M, Resistor_SMD:R_0603_1608Metric, F.Cu at (79.8, 40.7)
- added R1: 1M, Resistor_SMD:R_0603_1608Metric, F.Cu at (130.2, 91.1)
- added R1: 1M, Resistor_SMD:R_0603_1608Metric, F.Cu at (147.0, 107.9)
- added R1: 1M, Resistor_SMD:R_0603_1608Metric, F.Cu at (130.2, 74.3)
- added R1: 1M, Resistor_SMD:R_0603_1608Metric, F.Cu at (96.6, 40.7)
- added R1: 1M, Resistor_SMD:R_0603_1608Metric, F.Cu at (96.6, 107.9)
- added R1: 1M, Resistor_SMD:R_0603_1608Metric, F.Cu at (130.2, 57.5)
- added R1: 1M, Resistor_SMD:R_0603_1608Metric, F.Cu at (130.2, 107.9)
- added R1: 1M, Resistor_SMD:R_0603_1608Metric, F.Cu at (113.4, 74.3)
- added R1: 1M, Resistor_SMD:R_0603_1608Metric, F.Cu at (79.8, 74.3)
- added R1: 1M, Resistor_SMD:R_0603_1608Metric, F.Cu at (130.2, 40.7)
- added R1: 1M, Resistor_SMD:R_0603_1608Metric, F.Cu at (79.8, 107.9)
- added R1: 1M, Resistor_SMD:R_0603_1608Metric, F.Cu at (113.4, 40.7)
- added R1: 1M, Resistor_SMD:R_0603_1608Metric, F.Cu at (79.8, 91.1)
- added R1: 1M, Resistor_SMD:R_0603_1608Metric, F.Cu at (96.6, 57.5)
- added R1: 1M, Resistor_SMD:R_0603_1608Metric, F.Cu at (113.4, 91.1)
- added R1: 1M, Resistor_SMD:R_0603_1608Metric, F.Cu at (147.0, 40.7)
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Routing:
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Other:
- board text added: "LEDTreiber V1.1"
- board text removed: "LEDTreiber V1.0"
